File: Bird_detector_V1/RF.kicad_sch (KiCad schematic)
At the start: 64 parts, among them IC1 TXB0108PWR, J1 SIM_Card_Shielded, J2 GSM, J3 USB_A, J4 BT, J5 GNSS, Q1 SSM6N7002, Q2 SSM6N7002, Q3 SSM6N7002, Q4 SSM6N7002, Q5 SSM6N7002, SW1 SW_SPST, U1 SIM808

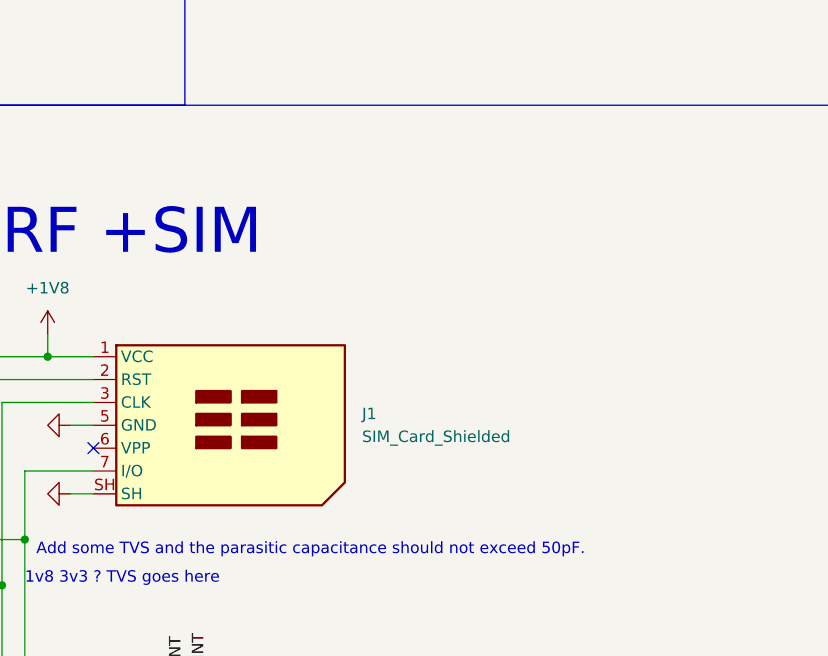
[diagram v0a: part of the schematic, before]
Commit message: K
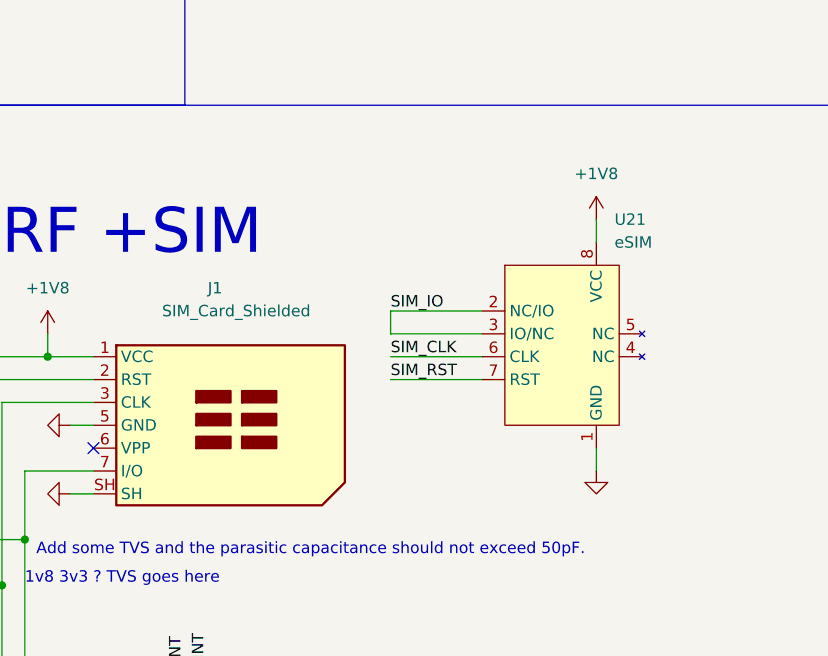
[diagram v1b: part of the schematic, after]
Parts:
- added U21: eSIM, Z_mycustom_footprint_lib:eSIM, symbol My_custom_lib:eSIM
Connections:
- net +1V8: now also U21.8 (VCC)
- net GND: now also U21.1 (GND)
- net SIM_CLK: now also U21.6 (CLK)
- net SIM_IO: now also U21.2 (NC/IO), U21.3 (IO/NC)
- net SIM_RST: now also U21.7 (RST)
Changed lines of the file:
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@@
+    (stroke (width 0) (type default) (color 0 0 0 0))
+  )
+  (wire (pts (xy 190.5 142.24) (xy 190.5 144.78))
     (stroke (width 0) (type default) (color 0 0 0 0))
   )
@@
     (stroke (width 0) (type default) (color 0 0 0 0))
   )
+  (wire (pts (xy 167.64 134.62) (xy 177.8 134.62))
+    (stroke (width 0) (type default) (color 0 0 0 0))
+  )
   (wire (pts (xy 109.22 139.7) (xy 109.22 142.24))
     (stroke (width 0) (type default) (color 0 0 0 0))
@@
     (stroke (width 0) (type default) (color 0 0 0 0))
   )
+  (wire (pts (xy 167.64 129.54) (xy 177.8 129.54))
+    (stroke (width 0) (type default) (color 0 0 0 0))
+  )
   (wire (pts (xy 93.98 182.88) (xy 93.98 180.34))
     (stroke (width 0) (type default) (color 0 0 0 0))
@@
     (stroke (width 0) (type default) (color 0 0 0 0))
   )
+  (wire (pts (xy 167.64 132.08) (xy 177.8 132.08))
+    (stroke (width 0) (type default) (color 0 0 0 0))
+  )
   (wire (pts (xy 269.24 193.04) (xy 269.24 195.58))
     (stroke (width 0) (type default) (color 0 0 0 0))
@@
     (stroke (width 0) (type default) (color 0 0 0 0))
   )
+  (wire (pts (xy 190.5 116.84) (xy 190.5 119.38))
+    (stroke (width 0) (type default) (color 0 0 0 0))
+  )
   (wire (pts (xy 345.44 236.22) (xy 345.44 238.76))
     (stroke (width 0) (type default) (color 0 0 0 0))
@@
     (stroke (width 0) (type default) (color 0 0 0 0))
   )
+  (wire (pts (xy 167.64 127) (xy 167.64 129.54))
+    (stroke (width 0) (type default) (color 0 0 0 0))
+  )
   (wire (pts (xy 266.7 182.88) (xy 278.13 182.88))
     (stroke (width 0) (type default) (color 0 0 0 0))
@@
   )
   (wire (pts (xy 322.58 220.98) (xy 322.58 223.52))
+    (stroke (width 0) (type default) (color 0 0 0 0))
+  )
+  (wire (pts (xy 167.64 127) (xy 177.8 127))
     (stroke (width 0) (type default) (color 0 0 0 0))
   )
@@
     (effects (font (size 1.27 1.27)) (justify left bottom))
   )
+  (label "SIM_RST" (at 167.64 134.62 0)
+    (effects (font (size 1.27 1.27)) (justify left bottom))
+  )
   (label "SIM_CLK" (at 106.68 157.48 0)
     (effects (font (size 1.27 1.27)) (justify left bottom))
@@
     (effects (font (size 1.27 1.27)) (justify right bottom))
   )
+  (label "SIM_IO" (at 167.64 127 0)
+    (effects (font (size 1.27 1.27)) (justify left bottom))
+  )
   (label "DTR" (at 43.18 180.34 0)
     (effects (font (size 1.27 1.27)) (justify left bottom))
@@
   )
   (label "BT_RF2" (at 203.2 238.76 0)
+    (effects (font (size 1.27 1.27)) (justify left bottom))
+  )
+  (label "SIM_CLK" (at 167.64 132.08 0)
     (effects (font (size 1.27 1.27)) (justify left bottom))
   )
@@
     (pin "1")
   )
+  (symbol (lib_id "My_custom_lib:eSIM") (at 187.96 127 0) (unit 1)
+    (in_bom yes) (on_board yes) (fields_autoplaced)
+    (property "Reference" "U21" (id 0) (at 192.5194 116.84 0)
+      (effects (font (size 1.27 1.27)) (justify left))
+    )
+    (property "Value" "eSIM" (id 1) (at 192.5194 119.38 0)
+      (effects (font (size 1.27 1.27)) (justify left))
+    )
+    (property "Footprint" "Z_mycustom_footprint_lib:eSIM" (id 2) (at 187.96 114.3 0)
+      (effects (font (size 1.27 1.27)) hide)
+    )
+    (property "Datasheet" "" (id 3) (at 187.96 114.3 0)
+      (effects (font (size 1.27 1.27)) hide)
+    )
+    (pin "1")
+    (pin "2")
+    (pin "3")
+    (pin "4")
+    (pin "5")
+    (pin "6")
+    (pin "7")
+    (pin "8")
+  )
   (symbol (lib_id "Connector:SIM_Card_Shielded") (at 147.32 139.7 0) (unit 1)
-    (in_bom yes) (on_board yes) (fields_autoplaced)
-    (property "Reference" "J1" (id 0) (at 164.465 138.4299 0)
-      (effects (font (size 1.27 1.27)) (justify left))
-    )
-    (property "Value" "SIM_Card_Shielded" (id 1) (at 164.465 140.9699 0)
+    (in_bom yes) (on_board yes)
+    (property "Reference" "J1" (id 0) (at 147.32 124.46 0)
+      (effects (font (size 1.27 1.27)) (justify left))
+    )
+    (property "Value" "SIM_Card_Shielded" (id 1) (at 142.24 127 0)
       (effects (font (size 1.27 1.27)) (justify left))
     )
@@
     )
     (property "Datasheet" "" (id 3) (at 383.54 220.98 0)
+      (effects (font (size 1.27 1.27)) hide)
+    )
+    (pin "1")
+  )
+  (symbol (lib_id "power:GND") (at 190.5 144.78 0) (unit 1)
+    (in_bom yes) (on_board yes) (fields_autoplaced)
+    (property "Reference" "#PWR0238" (id 0) (at 190.5 151.13 0)
+      (effects (font (size 1.27 1.27)) hide)
+    )
+    (property "Value" "GND" (id 1) (at 190.5 149.86 0)
+      (effects (font (size 1.27 1.27)) hide)
+    )
+    (property "Footprint" "" (id 2) (at 190.5 144.78 0)
+      (effects (font (size 1.27 1.27)) hide)
+    )
+    (property "Datasheet" "" (id 3) (at 190.5 144.78 0)
       (effects (font (size 1.27 1.27)) hide)
     )
@@
       (effects (font (size 1.27 1.27)) hide)
     )
+    (pin "1")
+  )
+  (symbol (lib_id "power:+1V8") (at 190.5 116.84 0) (unit 1)
+    (in_bom yes) (on_board yes) (fields_autoplaced)
+    (property "Reference" "#PWR0237" (id 0) (at 190.5 120.65 0)
+      (effects (font (size 1.27 1.27)) hide)
+    )
+    (property "Value" "+1V8" (id 1) (at 190.5 111.76 0))
+    (property "Footprint" "" (id 2) (at 190.5 116.84 0)
+      (effects (font (size 1.27 1.27)) hide)
+    )
+    (property "Datasheet" "" (id 3) (at 190.5 116.84 0)
+      (effects (font (size 1.27 1.27)) hide)
+    )
